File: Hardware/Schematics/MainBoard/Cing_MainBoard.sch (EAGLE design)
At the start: 178 parts, among them IC1 L293D, IC2 LM2576S, IC3 FT232RL, IC5 BME280, Q1 16mhz, Q2 BSS138, Q3 BSS138, Q4 BSS138, Q5 BSS138, Q6 NP2301AMR-G, Q7 NP2301AMR-G, U3 MPU-6050MPU6050

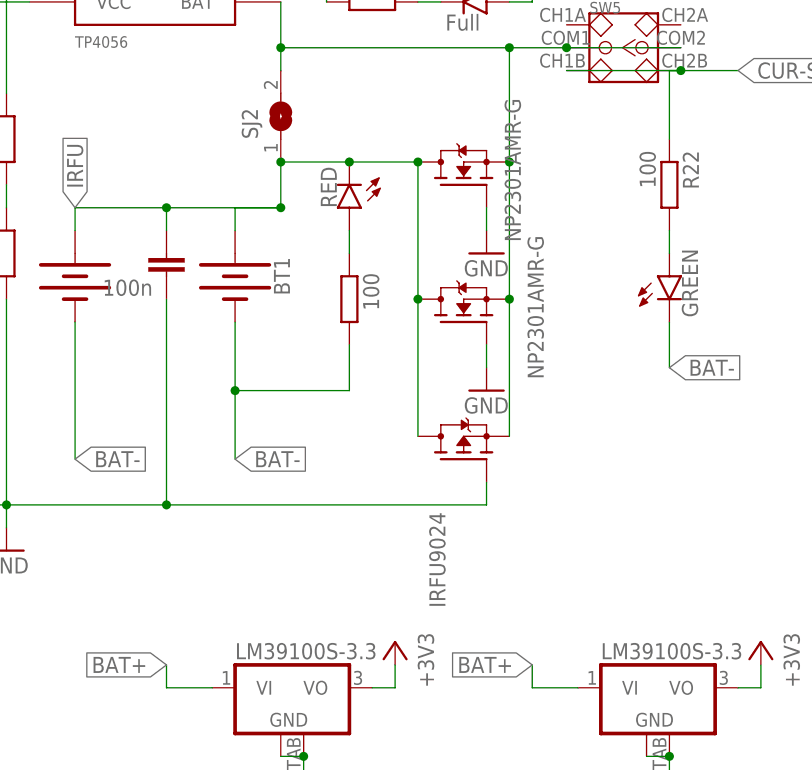
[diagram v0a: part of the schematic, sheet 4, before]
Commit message: commit
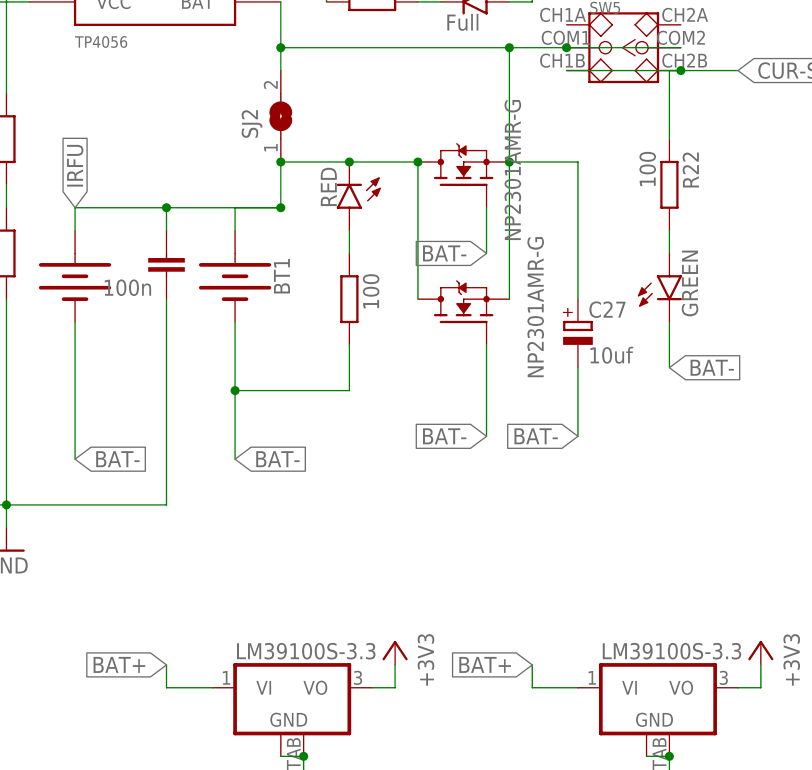
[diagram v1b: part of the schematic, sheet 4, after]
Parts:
- removed IRFU9024: IRFU9024, Cing Library:IRFU9024
- added C27: 10uf, rcl:CPOL-EU153CLV-0505
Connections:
- net BAT-: now also C27.-, Q6.G, Q7.G
- net GND: no longer IRFU9024.G, Q6.G, Q7.G
- net IRFU: no longer IRFU9024.D
- net N$26: now also C27.+; no longer IRFU9024.S
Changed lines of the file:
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@@
 <part name="U$4" library="Cing Library" library_urn="urn:adsk.eagle:library:10154637" deviceset="SERIAL_HEADER" device="" package3d_urn="urn:adsk.eagle:package:10154732/1" override_package3d_urn="urn:adsk.eagle:package:11838096/2" override_package_urn="urn:adsk.eagle:footprint:10154683/1"/>
 <part name="IC1" library="Cing Library" library_urn="urn:adsk.eagle:library:10154637" deviceset="L293D" device="" package3d_urn="urn:adsk.eagle:package:10154745/1" override_package3d_urn="urn:adsk.eagle:package:11833773/2" override_package_urn="urn:adsk.eagle:footprint:10154703/1" value="L293D  "/>
-<part name="IRFU9024" library="Cing Library" library_urn="urn:adsk.eagle:library:10154637" deviceset="IRFU9024" device="" package3d_urn="urn:adsk.eagle:package:10154729/1" override_package3d_urn="urn:adsk.eagle:package:11834780/2" override_package_urn="urn:adsk.eagle:footprint:10154686/1"/>
 <part name="U$7" library="Cing Library" library_urn="urn:adsk.eagle:library:10154637" deviceset="BATTERY_CONECTOR_D" device="" package3d_urn="urn:adsk.eagle:package:10154722/1" override_package3d_urn="urn:adsk.eagle:package:11838339/2" override_package_urn="urn:adsk.eagle:footprint:10154693/1"/>
 <part name="TP4056" library="Cing Library" library_urn="urn:adsk.eagle:library:10154637" deviceset="TP4056" device="" package3d_urn="urn:adsk.eagle:package:10154725/1" override_package3d_urn="urn:adsk.eagle:package:11834733/2" override_package_urn="urn:adsk.eagle:footprint:10154690/1"/>
@@
 <part name="GND48" library="supply1" library_urn="urn:adsk.eagle:library:371" deviceset="GND" device=""/>
 <part name="Q7" library="Cing Library" library_urn="urn:adsk.eagle:library:10154637" deviceset="NP2301AMR-G" device="" package3d_urn="urn:adsk.eagle:package:10154715/1" override_package3d_urn="urn:adsk.eagle:package:11834602/2" override_package_urn="urn:adsk.eagle:footprint:10154700/1" value="NP2301AMR-G"/>
-<part name="GND49" library="supply1" library_urn="urn:adsk.eagle:library:371" deviceset="GND" device=""/>
 <part name="Q6" library="Cing Library" library_urn="urn:adsk.eagle:library:10154637" deviceset="NP2301AMR-G" device="" package3d_urn="urn:adsk.eagle:package:10154715/1" override_package3d_urn="urn:adsk.eagle:package:11833702/2" override_package_urn="urn:adsk.eagle:footprint:10154700/1" value="NP2301AMR-G"/>
-<part name="GND61" library="supply1" library_urn="urn:adsk.eagle:library:371" deviceset="GND" device=""/>
 <part name="GND63" library="supply1" library_urn="urn:adsk.eagle:library:371" deviceset="GND" device=""/>
 <part name="+3V32" library="supply1" library_urn="urn:adsk.eagle:library:371" deviceset="+3V3" device=""/>
@@
 <part name="C25" library="rcl" library_urn="urn:adsk.eagle:library:334" deviceset="C-EU" device="C1206" package3d_urn="urn:adsk.eagle:package:23618/2" override_package3d_urn="urn:adsk.eagle:package:11833761/2" override_package_urn="urn:adsk.eagle:footprint:23125/1" value="100n"/>
 <part name="C26" library="rcl" library_urn="urn:adsk.eagle:library:334" deviceset="C-EU" device="C1206" package3d_urn="urn:adsk.eagle:package:23618/2" override_package3d_urn="urn:adsk.eagle:package:11833761/2" override_package_urn="urn:adsk.eagle:footprint:23125/1" value="100n"/>
+<part name="C27" library="rcl" library_urn="urn:adsk.eagle:library:334" deviceset="CPOL-EU" device="153CLV-0505" package3d_urn="urn:adsk.eagle:package:23402/2" value="10uf"/>
 </parts>
 <sheets>
@@
 <attribute name="VALUE" x="243.84" y="40.64" size="1.778" layer="96" rot="MR90"/>
 </instance>
-<instance part="IRFU9024" gate="G$1" x="208.28" y="66.04" smashed="yes" rot="MR90"/>
 <instance part="U$7" gate="G$1" x="165.1" y="86.36" smashed="yes" rot="R270"/>
 <instance part="TP4056" gate="G$1" x="165.1" y="127" smashed="yes">
@@
 <attribute name="VALUE" x="214.63" y="90.17" size="1.778" layer="96" rot="R90"/>
 </instance>
-<instance part="GND49" gate="1" x="210.82" y="88.9" smashed="yes">
-<attribute name="VALUE" x="208.28" y="86.36" size="1.778" layer="96"/>
-</instance>
 <instance part="Q6" gate="G$1" x="208.28" y="81.28" smashed="yes" rot="R90">
 <attribute name="VALUE" x="217.17" y="74.93" size="1.778" layer="96" rot="R90"/>
-</instance>
-<instance part="GND61" gate="1" x="210.82" y="73.66" smashed="yes">
-<attribute name="VALUE" x="208.28" y="71.12" size="1.778" layer="96"/>
 </instance>
 <instance part="U$25" gate="G$1" x="187.96" y="40.64" smashed="yes">
@@
 <instance part="GND64" gate="1" x="33.02" y="99.06" smashed="yes">
 <attribute name="VALUE" x="30.48" y="96.52" size="1.778" layer="96"/>
+</instance>
+<instance part="C27" gate="G$1" x="220.98" y="81.28" smashed="yes">
+<attribute name="NAME" x="222.123" y="81.7626" size="1.778" layer="95"/>
+<attribute name="VALUE" x="222.123" y="76.6826" size="1.778" layer="96"/>
 </instance>
 </instances>
@@
 </segment>
 <segment>
-<wire x1="175.26" y1="60.96" x2="210.82" y2="60.96" width="0.1524" layer="91"/>
-<wire x1="210.82" y1="63.5" x2="210.82" y2="60.96" width="0.1524" layer="91"/>
 <pinref part="C1" gate="G$1" pin="2"/>
 <wire x1="175.26" y1="83.82" x2="175.26" y2="60.96" width="0.1524" layer="91"/>
@@
 <wire x1="149.86" y1="60.96" x2="157.48" y2="60.96" width="0.1524" layer="91"/>
 <junction x="149.86" y="119.38"/>
-<junction x="175.26" y="60.96"/>
 <wire x1="157.48" y1="60.96" x2="175.26" y2="60.96" width="0.1524" layer="91"/>
 <junction x="157.48" y="60.96"/>
 <pinref part="GND15" gate="1" pin="GND"/>
 <wire x1="157.48" y1="60.96" x2="157.48" y2="58.42" width="0.1524" layer="91"/>
-<pinref part="IRFU9024" gate="G$1" pin="G"/>
 <pinref part="TP4056" gate="G$1" pin="TEMP"/>
 <pinref part="TP4056" gate="G$1" pin="GND"/>
@@
 </segment>
 <segment>
-<pinref part="Q7" gate="G$1" pin="G"/>
-<pinref part="GND49" gate="1" pin="GND"/>
-<wire x1="210.82" y1="91.44" x2="210.82" y2="93.98" width="0.1524" layer="91"/>
-</segment>
-<segment>
-<pinref part="Q6" gate="G$1" pin="G"/>
-<pinref part="GND61" gate="1" pin="GND"/>
-<wire x1="210.82" y1="76.2" x2="210.82" y2="78.74" width="0.1524" layer="91"/>
-</segment>
-<segment>
 <pinref part="C4" gate="G$1" pin="2"/>
 <pinref part="GND37" gate="1" pin="GND"/>
@@
 <wire x1="182.88" y1="93.98" x2="187.96" y2="93.98" width="0.1524" layer="91"/>
 <junction x="175.26" y="93.98"/>
-<pinref part="IRFU9024" gate="G$1" pin="D"/>
 <pinref part="U$7" gate="G$1" pin="+"/>
 <wire x1="187.96" y1="93.98" x2="175.26" y2="93.98" width="0.1524" layer="91"/>
@@
 <wire x1="187.96" y1="99.06" x2="187.96" y2="93.98" width="0.1524" layer="91"/>
 <wire x1="195.58" y1="99.06" x2="187.96" y2="99.06" width="0.1524" layer="91"/>
-<wire x1="203.2" y1="68.58" x2="203.2" y2="83.82" width="0.1524" layer="91"/>
 <wire x1="203.2" y1="83.82" x2="203.2" y2="99.06" width="0.1524" layer="91"/>
 <wire x1="203.2" y1="99.06" x2="195.58" y2="99.06" width="0.1524" layer="91"/>
@@
 <junction x="203.2" y="99.06"/>
 <pinref part="Q6" gate="G$1" pin="D"/>
-<junction x="203.2" y="83.82"/>
 </segment>
 </net>
@@
 <wire x1="219.71" y1="111.76" x2="213.36" y2="111.76" width="0.1524" layer="91"/>
 <junction x="219.71" y="111.76"/>
-<wire x1="213.36" y1="68.58" x2="213.36" y2="83.82" width="0.1524" layer="91"/>
-<pinref part="IRFU9024" gate="G$1" pin="S"/>
 <pinref part="TP4056" gate="G$1" pin="BAT"/>
 <wire x1="213.36" y1="83.82" x2="213.36" y2="99.06" width="0.1524" layer="91"/>
@@
 <junction x="213.36" y="99.06"/>
 <pinref part="Q6" gate="G$1" pin="S"/>
-<junction x="213.36" y="83.82"/>
+<pinref part="C27" gate="G$1" pin="+"/>
+<wire x1="220.98" y1="83.82" x2="220.98" y2="99.06" width="0.1524" layer="91"/>
+<wire x1="220.98" y1="99.06" x2="213.36" y2="99.06" width="0.1524" layer="91"/>
 </segment>
 </net>
@@
 <label x="231.14" y="76.2" size="1.778" layer="95" xref="yes"/>
 </segment>
-</net>
+<segment>
+<wire x1="210.82" y1="78.74" x2="210.82" y2="68.58" width="0.1524" layer="91"/>
+<pinref part="Q6" gate="G$1" pin="G"/>
+<label x="210.82" y="68.58" size="1.778" layer="95" rot="R180" xref="yes"/>
+</segment>
+<segment>
+<wire x1="220.98" y1="76.2" x2="220.98" y2="68.58" width="0.1524" layer="91"/>
+<pinref part="C27" gate="G$1" pin="-"/>
+<label x="220.98" y="68.58" size="1.778" layer="95" rot="R180" xref="yes"/>
+</segment>
+<segment>
+<wire x1="210.82" y1="93.98" x2="210.82" y2="88.9" width="0.1524" layer="91"/>
+<pinref part="Q7" gate="G$1" pin="G"/>
+<label x="210.82" y="88.9" size="1.778" layer="95" rot="R180" xref="yes"/>
+</segment>
+</net>
